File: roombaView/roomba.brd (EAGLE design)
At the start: 57 x 34.1 mm, 15 parts

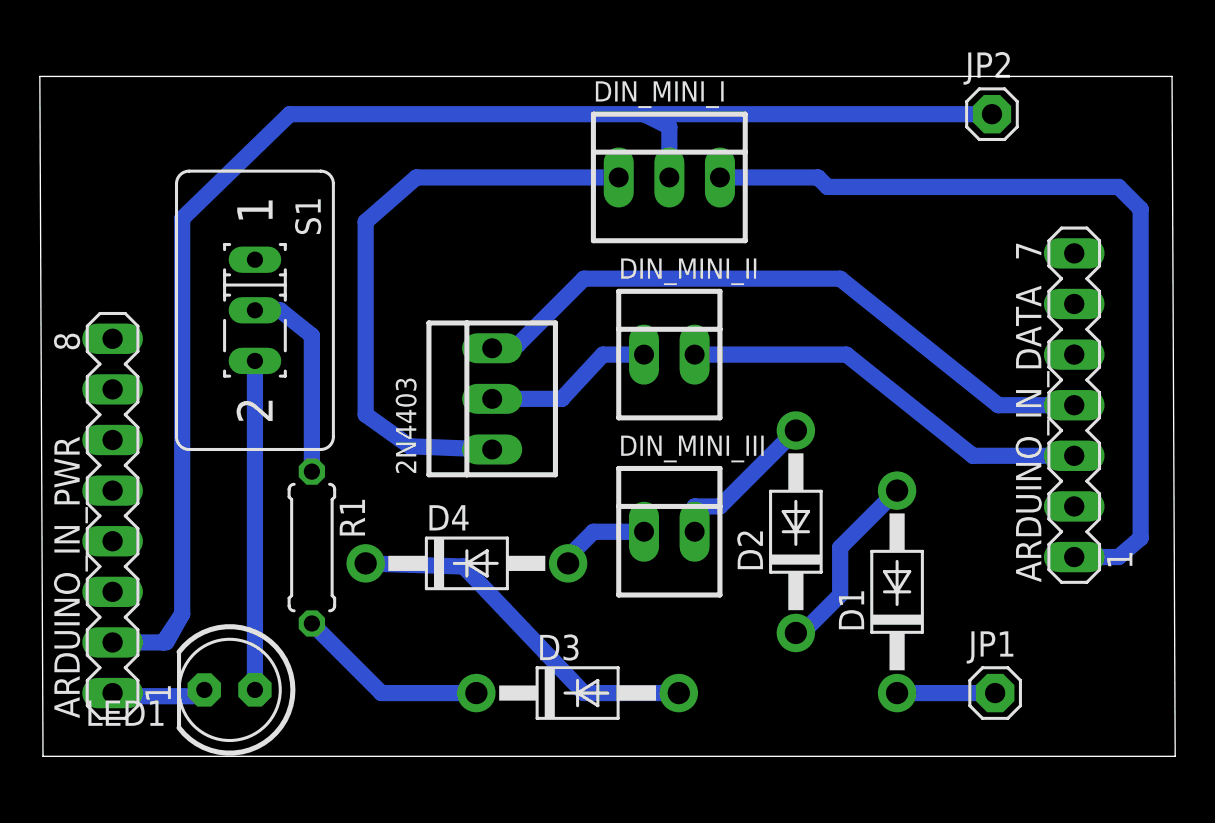
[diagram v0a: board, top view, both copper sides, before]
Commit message: update board
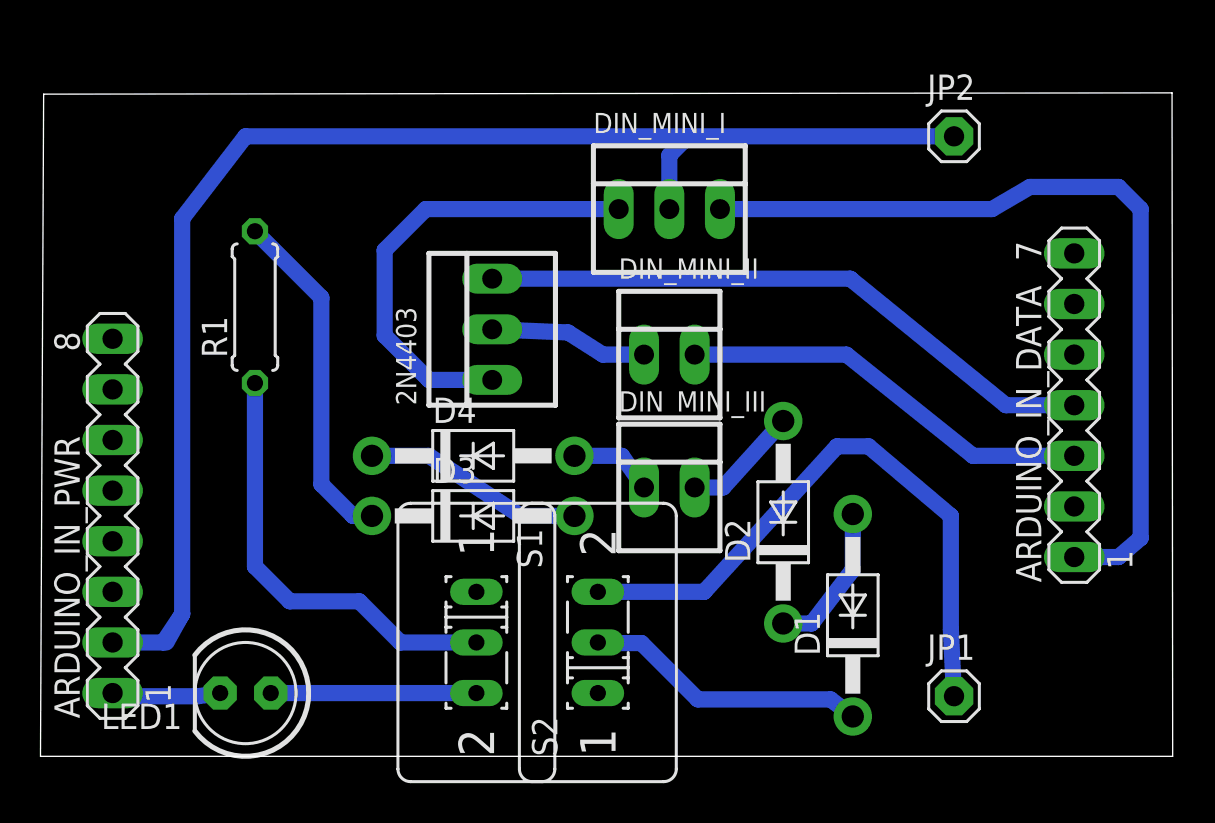
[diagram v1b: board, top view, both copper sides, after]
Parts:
- added S2: (no value), switch:M251
- moved S1 20.0 mm to (21.9, 5.71)
- moved R1 12.4 mm to (10.8, 22.5), turned to 90 degrees
- moved D3 10.3 mm to (21.7, 12.1)
- moved D4 5.41 mm to (21.7, 15.1)
- moved 2N4403 3.49 mm to (22.7, 21.4)
- moved D1 2.51 mm to (40.8, 7.08)
- moved DIN_MINI_III 2.22 mm to (31.6, 13.5)
- moved JP2 2.21 mm to (45.9, 31.1)
- moved JP1 2.07 mm to (45.9, 3.02)
- moved DIN_MINI_I 1.59 mm to (31.6, 27.5)
- moved LED1 0.81 mm to (10.3, 3.17)
- moved D2 0.79 mm to (37.3, 11.7)
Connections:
- new net N$16: JP1.1, S2.3
- net N$14: now also S2.2; no longer JP1.1
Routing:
- net N$16: track 0.00 -> 31.3 mm
- net N$3: track 10.1 -> 21.9 mm
- net N$14: track 4.92 -> 14.3 mm
- net N$15: track 9.70 -> 17.3 mm
- net N$4: track 18.4 -> 11.1 mm
- net N$2: track 30.1 -> 23.2 mm
- net N$12: track 16.5 -> 10.3 mm
- net N$10: track 7.93 -> 5.92 mm
- net N$5: track 72.5 -> 70.5 mm
- net N$11: track 9.43 -> 7.62 mm
- net N$6: track 32.9 -> 31.5 mm
- net N$13: track 4.80 -> 5.47 mm
- net N$1: track 8.59 -> 7.95 mm
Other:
- board size 57 x 34.1 mm -> 56.8 x 33.3 mm
